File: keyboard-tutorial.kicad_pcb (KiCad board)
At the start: 2 copper layers, 24 parts, among them SW1 SW_Push, U1 ATmega32U4-A, Y1 16MHz

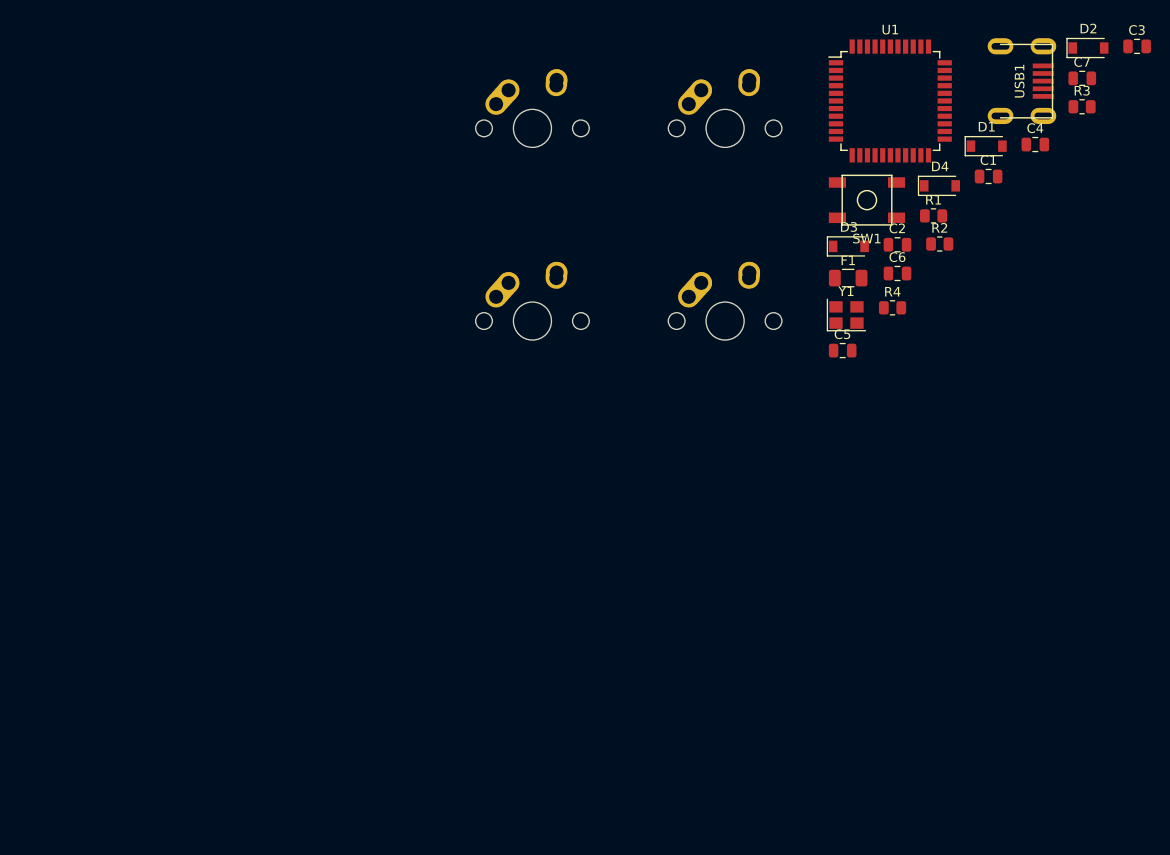
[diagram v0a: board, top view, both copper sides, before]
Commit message: Keyboard settings updates
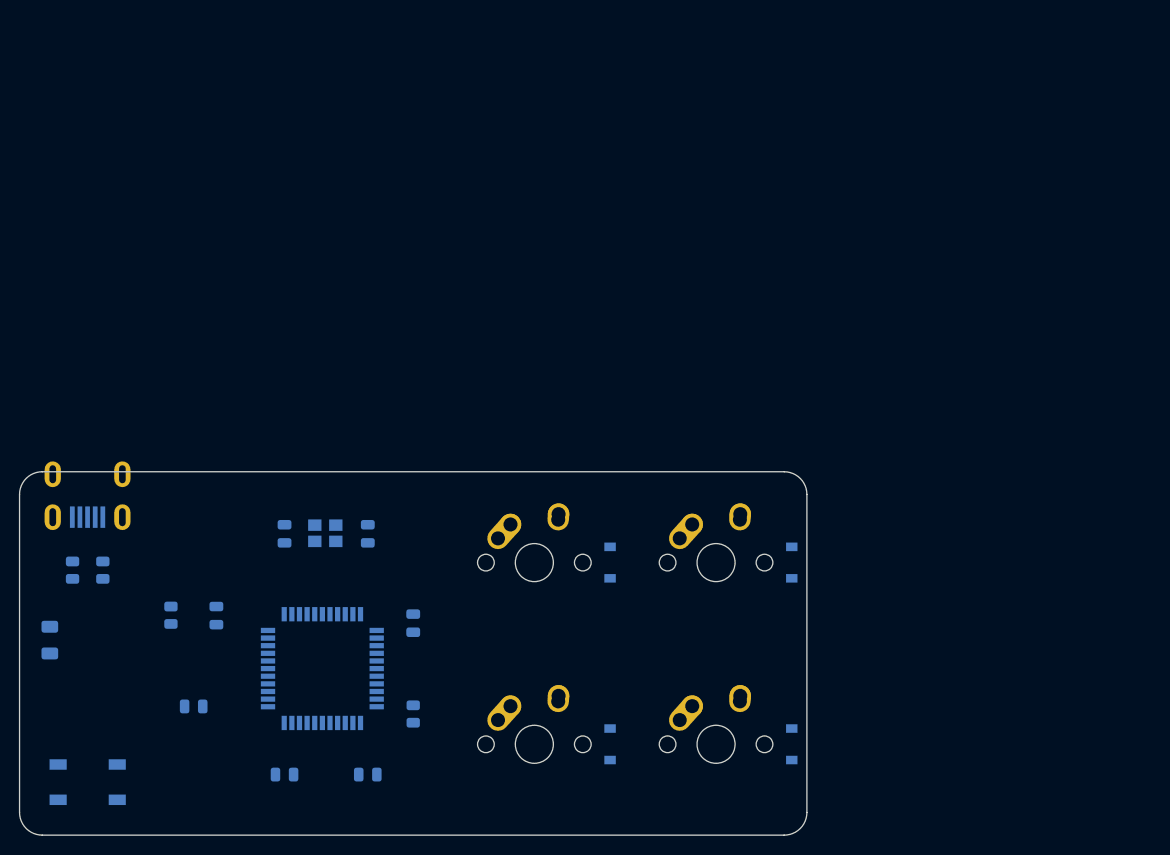
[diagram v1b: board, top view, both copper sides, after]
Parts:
- C1, C2, C3, C4, C5, C6, C7, D1, D2, D3, D4, F1, R1, R2, R3, R4, SW1, U1, USB1, Y1: moved to B.Cu
- moved C7 111.0 mm to (97.6, 139.7)
- moved R3 109.4 mm to (85.7, 123.0), turned to 90 degrees
- moved USB1 104.2 mm to (77.0, 108.2), turned to -90 degrees
- moved SW1 102.0 mm to (77.0, 140.5), turned to 180 degrees
- moved R1 97.6 mm to (75.4, 118.3), turned to -90 degrees
- moved C3 95.5 mm to (106.4, 114.5), turned to -90 degrees
- moved R2 94.2 mm to (78.6, 118.3), turned to -90 degrees
- moved C1 93.1 mm to (90.5, 123.0), turned to 90 degrees
- moved F1 91.9 mm to (73.0, 125.6), turned to -90 degrees
- moved C4 88.7 mm to (97.6, 114.5), turned to 90 degrees
- moved D2 88.6 mm to (131.8, 136.5), turned to 90 degrees
- moved C6 86.6 mm to (88.1, 132.6), turned to 180 degrees
- moved U1 84.2 mm to (101.6, 128.6)
- moved C2 78.5 mm to (106.4, 139.7), turned to 180 degrees
- moved R4 65.9 mm to (111.1, 133.3), turned to -90 degrees
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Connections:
- USB1 pad 3: unconnected-(USB1-Pad3) -> D+
- USB1 pad 4: D+ -> D-
- USB1 pad 5: D- -> VCC
- USB1 pad 6: VCC -> unconnected-(USB1-Pad6)
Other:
- board outline added: 82.6 x 38.1 mm
